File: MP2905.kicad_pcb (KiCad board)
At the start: 2 copper layers, 45 x 36.5 mm, 28 parts, among them Q1 NMOS, Q2 NMOS, Q3 NMOS, SW1 SW_Nidec_CAS-120A1, U1 MP2905EK-LF-P

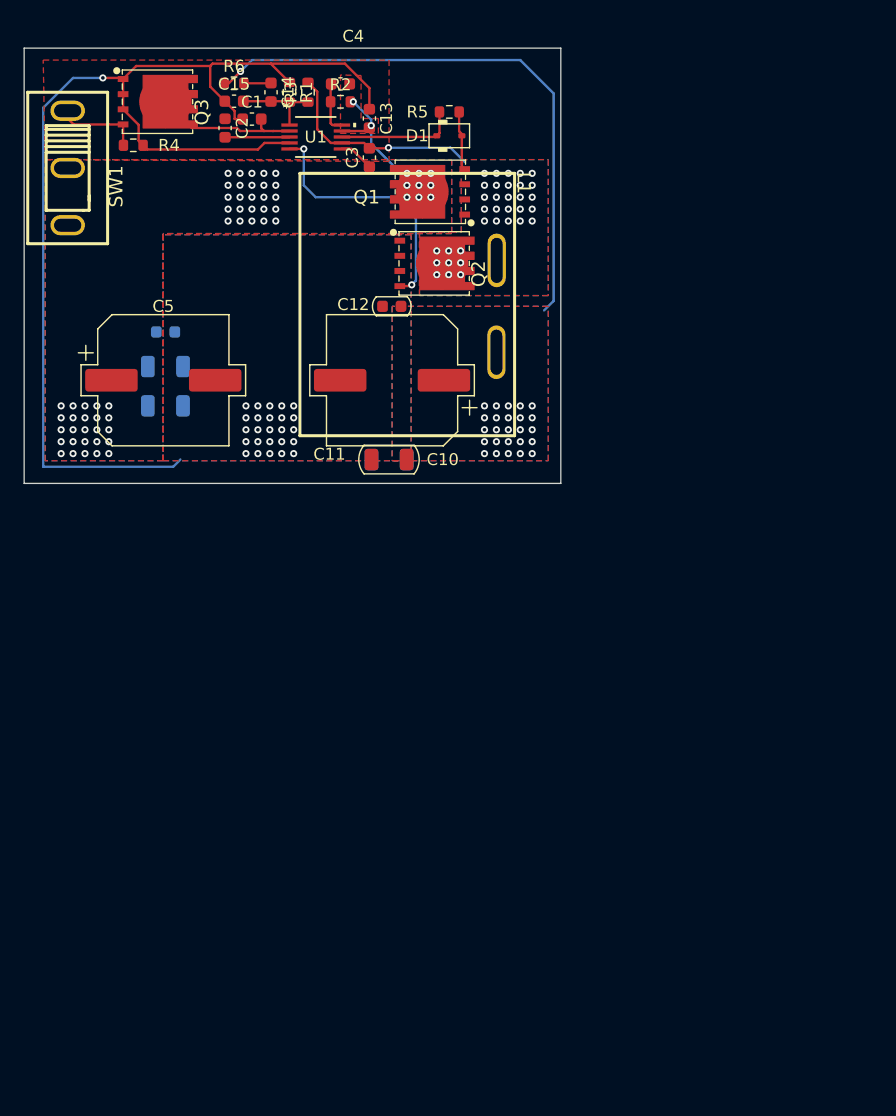
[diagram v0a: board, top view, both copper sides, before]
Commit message: 四层板
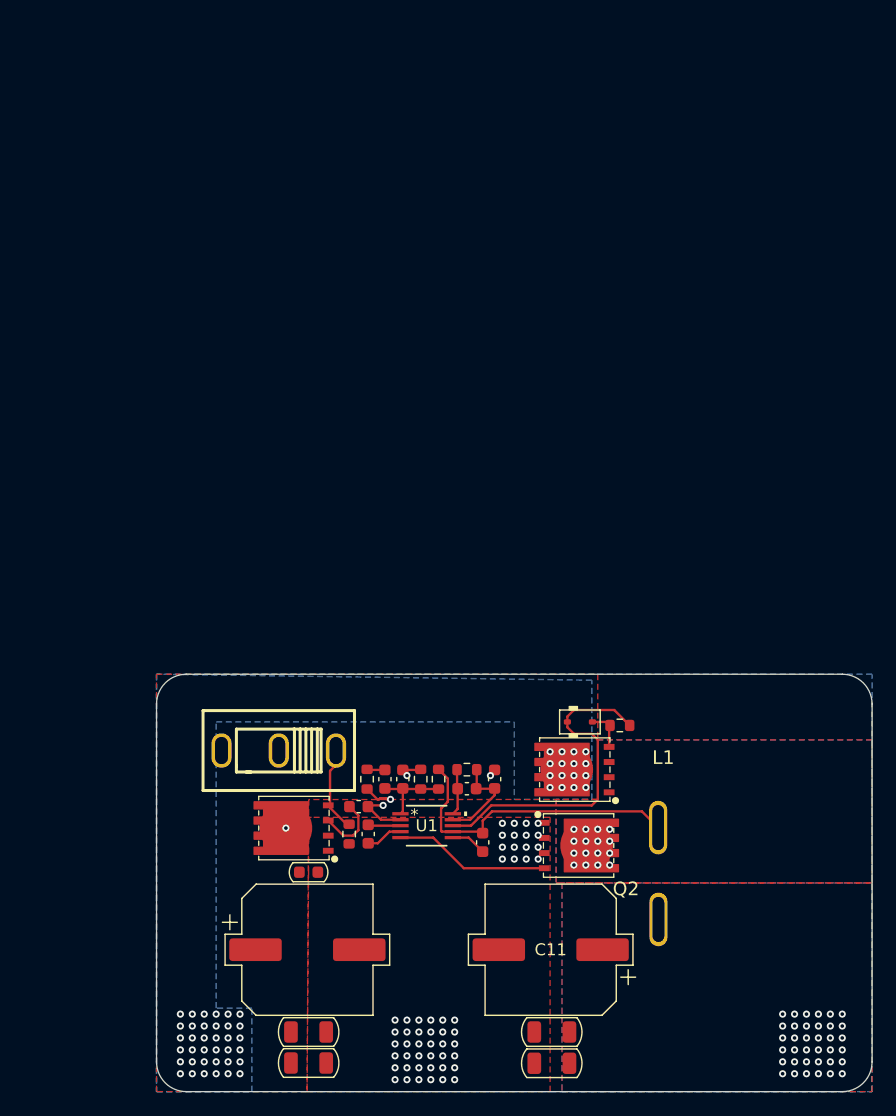
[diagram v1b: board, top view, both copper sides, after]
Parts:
- removed C12: C_0603, PCM_Capacitor_SMD_AKL:C_0603_1608Metric
- C10: value C_1206 -> 100UF
- C11: value CP_SMD_D10.0mm_H7.7mm -> 470uF
- C5: value CP_SMD_D10.0mm_H7.7mm -> 470UF
- C6: value C_0603 -> 10NF; moved to F.Cu
- C7, C8: value C_1206 -> 4.7UF; moved to F.Cu
- C9: value C_1206 -> 100UF; moved to F.Cu
- L1: moved to B.Cu
- R1: value R -> 1K
- R3: value R -> 2K
- R4: value R -> 20K
- R6: value 3K -> 10R
- moved Q3 62.4 mm to (91.2, 109.0), turned to 90 degrees
- moved R4 60.5 mm to (94.8, 109.5), turned to 90 degrees
- moved C2 60.4 mm to (96.3, 109.5), turned to 90 degrees
- moved C4 60.0 mm to (104.6, 105.7)
- moved C8 59.6 mm to (91.3, 128.7)
- moved R6 59.4 mm to (96.3, 104.9), turned to 90 degrees
- moved R1 58.6 mm to (100.8, 104.9)
- moved R3 58.6 mm to (102.2, 104.9)
- moved C15 58.6 mm to (99.3, 104.9), turned to -90 degrees
- moved U1 58.5 mm to (101.2, 108.8)
- moved C14 58.4 mm to (97.8, 104.9)
- moved C1 58.3 mm to (95.5, 107.2)
- moved C3 58.2 mm to (106.0, 110.2)
- moved R2 57.0 mm to (104.6, 104.1)
- moved C13 56.4 mm to (107.0, 104.9)
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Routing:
- net GND: track 100.5 -> 10.2 mm, vias 26 -> 54
- net /VOUT: track 48.1 -> 23.8 mm, vias 26 -> 37
- net /HG: track 10.1 -> 27.9 mm
- net /LG: track 21.5 -> 13.1 mm, vias 2 -> 0
- net /SW: track 17.8 -> 25.9 mm, vias 35 -> 16
- net Net-(U1-REF): track 5.41 -> 2.73 mm
- net +12V: track 10.6 -> 8.11 mm, vias 61 -> 52
- net Net-(D1-A): track 5.14 -> 3.42 mm
- net Net-(C14-Pad1): track 2.29 -> 1.52 mm
- net Net-(U1-FB): track 7.39 -> 6.72 mm
- net Net-(Q3-D): track 13.5 -> 13.4 mm, vias 0 -> 2
- added copper zone on In1.Cu, net +12V
- added copper zone on In2.Cu, net +12V
- added copper zone on In1.Cu, net /SW
- added copper zone on In2.Cu, net /SW
- added copper zone on In1.Cu, net /VOUT
- added copper zone on In2.Cu, net /VOUT
- added copper zone on In1.Cu, net GND
- added copper zone on In2.Cu, net GND
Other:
- board size 45 x 36.5 mm -> 60 x 35 mm
- copper layers 2 -> 4
